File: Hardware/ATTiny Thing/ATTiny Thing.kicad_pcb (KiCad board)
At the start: 2 copper layers, 30 x 14 mm, 12 parts, among them J1 JST_SH_BM048, J2 UPDI Connection, U1 ATtiny1617

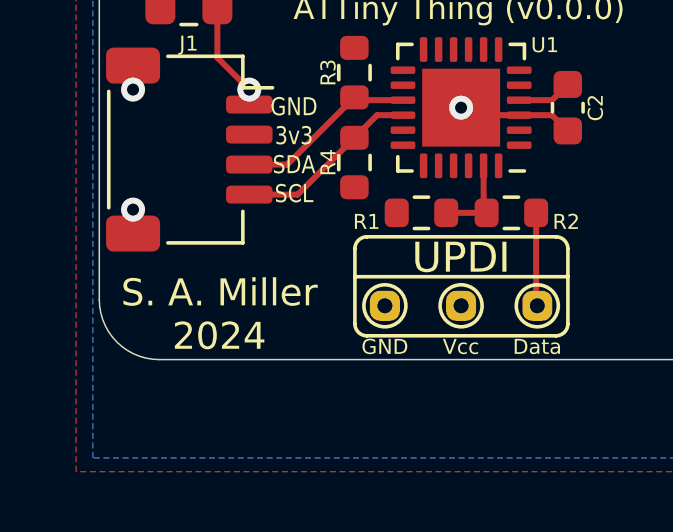
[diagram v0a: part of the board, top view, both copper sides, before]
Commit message: ...
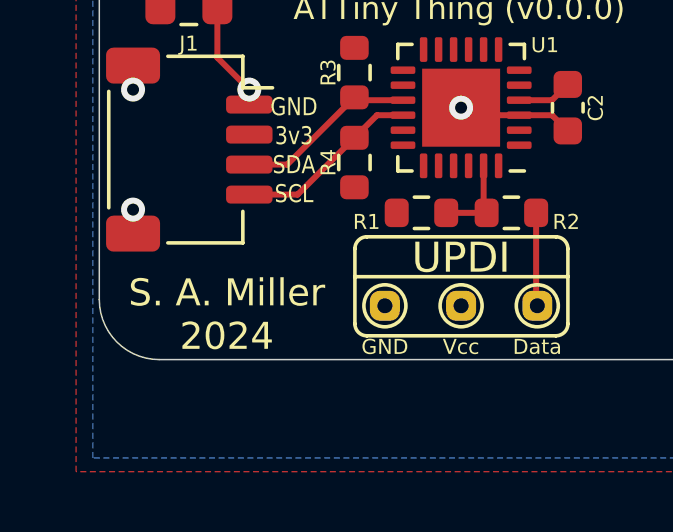
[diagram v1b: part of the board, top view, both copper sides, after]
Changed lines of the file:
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@@
     (effects (font (size 0.9 0.9) (thickness 0.15)))
   )
-  (gr_text "${COMPANY}\n${ISSUE_DATE}" (at 89 105.5) (layer "F.SilkS")
+  (gr_text "${COMPANY}\n${ISSUE_DATE}" (at 89.25 105.5) (layer "F.SilkS")
     (effects (font (size 0.9 0.9) (thickness 0.15)))
   )
